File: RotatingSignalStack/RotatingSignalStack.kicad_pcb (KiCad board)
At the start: 2 copper layers, 66.5 x 56.4 mm, 96 parts, among them IC2 STM32H562RIT6, J1 Conn_01x06, J2 Conn_01x04, J3 RJ45_LED_Shielded, J4 Conn_01x09, SW1 SW_Push, SW2 Boot Switch, SW5 SW_Push, SW6 SW_Push, SW7 SW_Push, T1 GMG116S1202R, U1 TMAG5273C1QDBVR, U2 AP63203WU-7, U3 SN65HVD232, U4 DP83825I, U5 SG-210STF 50.0000ML0, U6 USBLC6-2SC6, U7 USBLC6-4SC6, U8 OKI-78SR-3.3_1.5-W36-C

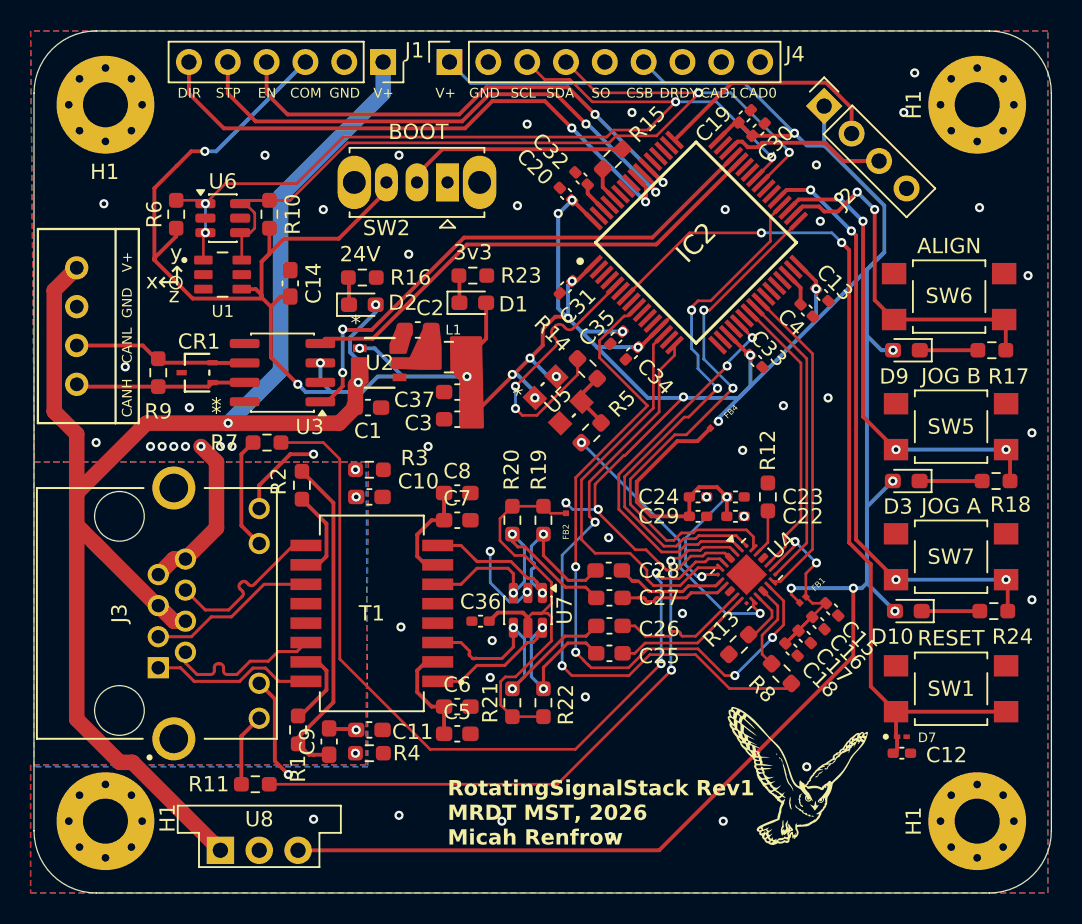
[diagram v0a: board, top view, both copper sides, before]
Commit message: final layout
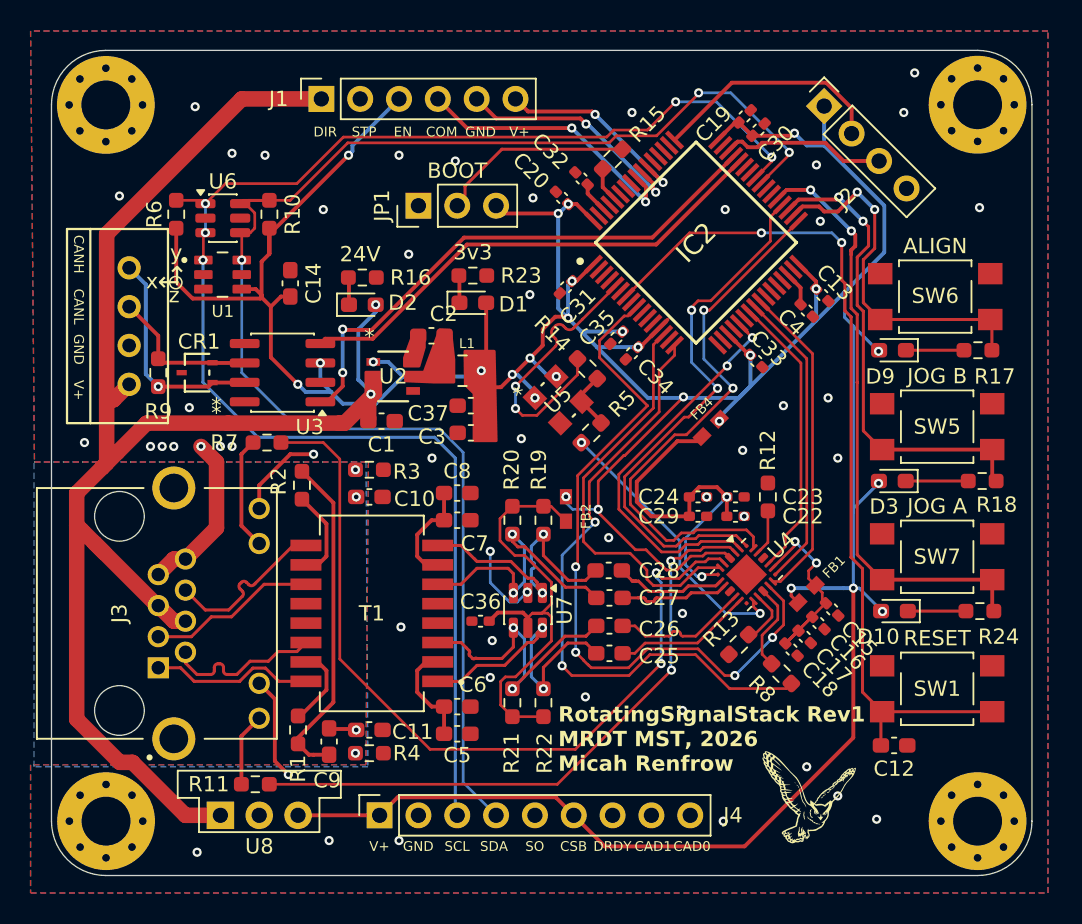
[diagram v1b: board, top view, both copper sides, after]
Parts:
- removed D7: ESDALC6V1-1U2, SignalStack:DIODE_ESDALC6V1-1U2
- removed the H1 at (185.9, 105.5)
- removed the H1 at (128.9, 105.5)
- removed the H1 at (128.9, 58.7)
- removed SW2: Boot Switch, Button_Switch_THT:SW_Slide_SPDT_Straight_CK_OS102011MS2Q
- added H2: MountingHole, MountingHole:MountingHole_3.2mm_M3_Pad_Via, F.Cu at (128.9, 105.5)
- added H3: MountingHole, MountingHole:MountingHole_3.2mm_M3_Pad_Via, F.Cu at (128.9, 58.7)
- added H4: MountingHole, MountingHole:MountingHole_3.2mm_M3_Pad_Via, F.Cu at (185.9, 105.5)
- added JP1: Jumper_3_Bridged12, Connector_PinHeader_2.54mm:PinHeader_1x03_P2.54mm_Vertical, F.Cu at (149.4, 65.3)
- C12: footprint Capacitor_SMD:C_0402_1005Metric_Pad0.74x0.62mm_HandSolder -> Capacitor_SMD:C_0603_1608Metric_Pad1.08x0.95mm_HandSolder
- FB1, FB2, FB4: footprint SignalStack:BEADC0603X33N -> SignalStack:FB_MI0603L221R-10
- moved J4 49.5 mm to (146.8, 105.2)
- moved Conn1 8.36 mm to (130.4, 77.0), turned to 90 degrees
- moved J1 4.70 mm to (143.0, 58.3), turned to 90 degrees
- moved U8 2.29 mm to (136.4, 105.2)
- moved C3 1.26 mm to (152.8, 80.1)
- moved C37 1.26 mm to (152.8, 78.4)
- moved L1 1.26 mm to (152.2, 76.1)
- moved U2 1.26 mm to (147.7, 76.4)
- moved C1 1.26 mm to (146.9, 79.4)
- moved C2 0.97 mm to (150.2, 73.8)
- moved D10 0.91 mm to (180.5, 91.8)
- moved D9 0.91 mm to (180.4, 74.7)
- moved R24 0.91 mm to (186.1, 91.8)
- moved SW6 0.91 mm to (183.2, 71.2)
- moved D3 0.91 mm to (180.3, 83.3)
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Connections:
- H1 pad 1: (no net) -> GND
- IC2 pad 54: EN -> DIR
- IC2 pad 56: DIR -> EN
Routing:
- net +3V3: track 307.7 -> 265.9 mm
- net SCL: track 59.6 -> 98.8 mm, vias 4 -> 5
- net SDA: track 59.7 -> 98.8 mm, vias 2 -> 3
- net DIR: track 38.2 -> 13.3 mm
- net STP: track 35.9 -> 15.9 mm
- net EN: track 33.3 -> 18.2 mm
- net VBUS: track 111.7 -> 101.0 mm, vias 3 -> 2
- net /CAN/CANH: track 11.2 -> 14.3 mm, vias 0 -> 1
- net Net-(JP1-C): track 14.6 -> 11.9 mm
- net /CAN/CANL: track 11.5 -> 10.1 mm
- net Net-(IC2-NRST): track 58.3 -> 57.3 mm
- net Net-(U4-VDDA3V3): track 25.0 -> 24.2 mm
- net Net-(U4-VDDIO): track 15.7 -> 15.0 mm
- net /Buttons/JOG B: track 31.1 -> 31.7 mm, vias 4 -> 2
- net /Buttons/JOG A: vias 4 -> 2
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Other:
- board size 66.5 x 56.4 mm -> 64.1 x 54 mm
